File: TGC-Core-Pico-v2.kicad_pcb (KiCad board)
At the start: 4 copper layers, 37.6 x 63.1 mm, 36 parts, among them J2 Conn_01x18, J3 Conn_01x18, P1 USB_C_Plug_USB2.0, SW1 SW_Push, U1 RP2040, U2 AMS1117-3.3, U3 W25Q128JVS, U4 ESP32-C6-MINI-1, U5 SHT31-DIS, U6 ICM-20602, Y1 ABM8-272-T3

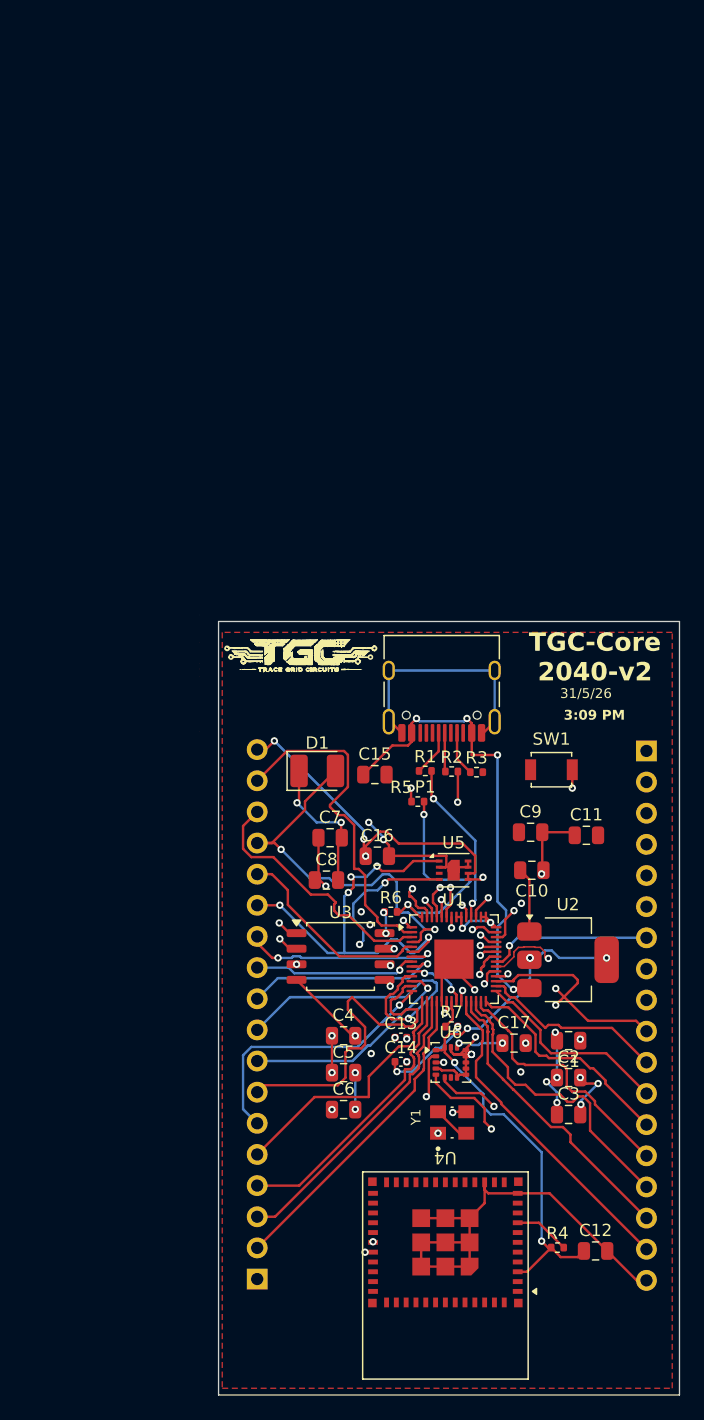
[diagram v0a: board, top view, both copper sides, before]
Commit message: Add files via upload
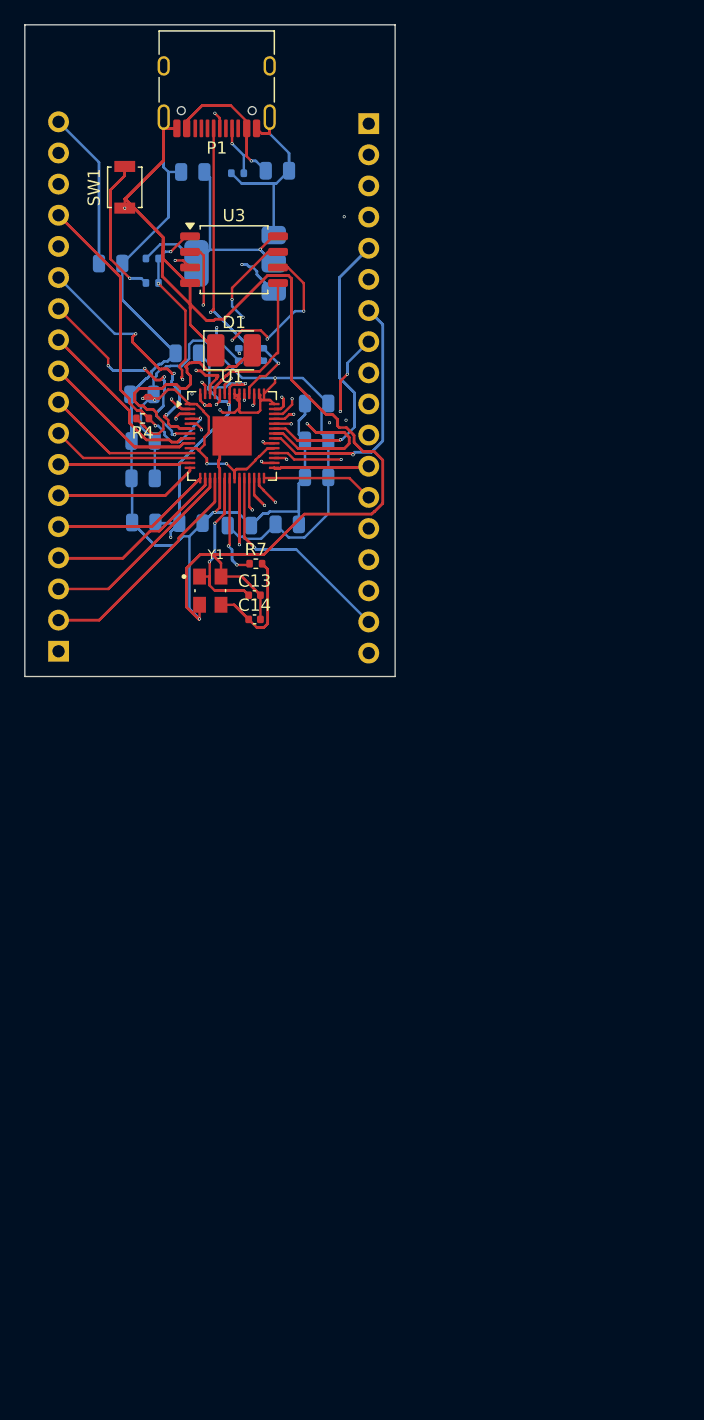
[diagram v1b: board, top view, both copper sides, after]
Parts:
- removed C17: 100nF, Capacitor_SMD:C_0805_2012Metric
- removed U4: ESP32-C6-MINI-1, RF_Module:ESP32-C6-MINI-1
- removed U5: SHT31-DIS, Sensor_Humidity:Sensirion_DFN-8-1EP_2.5x2.5mm_P0.5mm_EP1.1x1.7mm
- removed U6: ICM-20602, Package_LGA:LGA-16_3x3mm_P0.5mm_LayoutBorder3x5y
- C1, C10, C11, C12, C15, C16, C2, C3, C4, C5, C6, C7, C8, C9, R1, R2, R3, R5, R6, U2: moved to B.Cu
- R4: value 10k -> 220R
- moved C12 93.9 mm to (149.7, 37.3), turned to 180 degrees
- moved R4 75.6 mm to (145.6, 57.4), turned to 180 degrees
- moved U2 63.0 mm to (153.2, 44.8), turned to 180 degrees
- moved C3 61.5 mm to (159.8, 56.2), turned to 180 degrees
- moved C6 60.6 mm to (145.6, 55.4), turned to 180 degrees
- moved SW1 58.9 mm to (144.2, 38.5), turned to 90 degrees
- moved U3 57.5 mm to (153.1, 44.5)
- moved R6 56.7 mm to (146.4, 44.4)
- moved J2 55.9 mm to (164.1, 33.4)
- moved J3 53.7 mm to (138.8, 76.4)
- moved C16 53.0 mm to (143.0, 44.8)
- moved P1 52.6 mm to (151.7, 29.7)
- moved R3 52.6 mm to (153.3, 37.4), turned to 180 degrees
- moved C2 52.4 mm to (153.5, 66.1)
- moved C11 51.0 mm to (149.2, 52.1), turned to 180 degrees
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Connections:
- D1 pad 2: /GPIO2 -> Net-(D1-Pad2)
- R4 pad 1: +3.3V -> /GPIO2
- R4 pad 2: Net-(U4-EN) -> Net-(D1-Pad2)
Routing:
- net GND: track 163.6 -> 431.3 mm, vias 20 -> 3
- net /GPIO27_ADC1: track 19.3 -> 63.9 mm
- net /GPIO20: track 55.1 -> 13.9 mm, vias 3 -> 1
- net /D+: track 3.17 -> 40.9 mm, vias 0 -> 2
- net Net-(D1-Pad2): track 0.00 -> 35.7 mm
- net +1V1: track 28.7 -> 63.0 mm, vias 4 -> 5
- net /GPIO28_ADC2: track 18.8 -> 49.8 mm
- net /GPIO17: track 38.5 -> 9.20 mm, vias 1 -> 0
- net /GPIO26_ADC0: track 19.0 -> 47.2 mm, vias 1 -> 3
- net /GPIO23: track 13.5 -> 39.7 mm
- net /GPIO19: track 36.9 -> 10.7 mm
- net /GPIO25: track 18.0 -> 43.1 mm
- net /D-: track 3.76 -> 27.3 mm, vias 0 -> 1
- net /GPIO7: track 16.5 -> 38.7 mm, vias 1 -> 0
- net /GPIO24: track 19.6 -> 39.1 mm
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- removed copper zone on F.Cu, net GND
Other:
- board size 37.6 x 63.1 mm -> 30.2 x 53.2 mm
- board text removed: "31/5/26"
- board text removed: "3:09 PM"
- board text removed: "TGC-Core 2040-v2"
